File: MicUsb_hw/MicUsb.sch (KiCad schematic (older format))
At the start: 29 parts

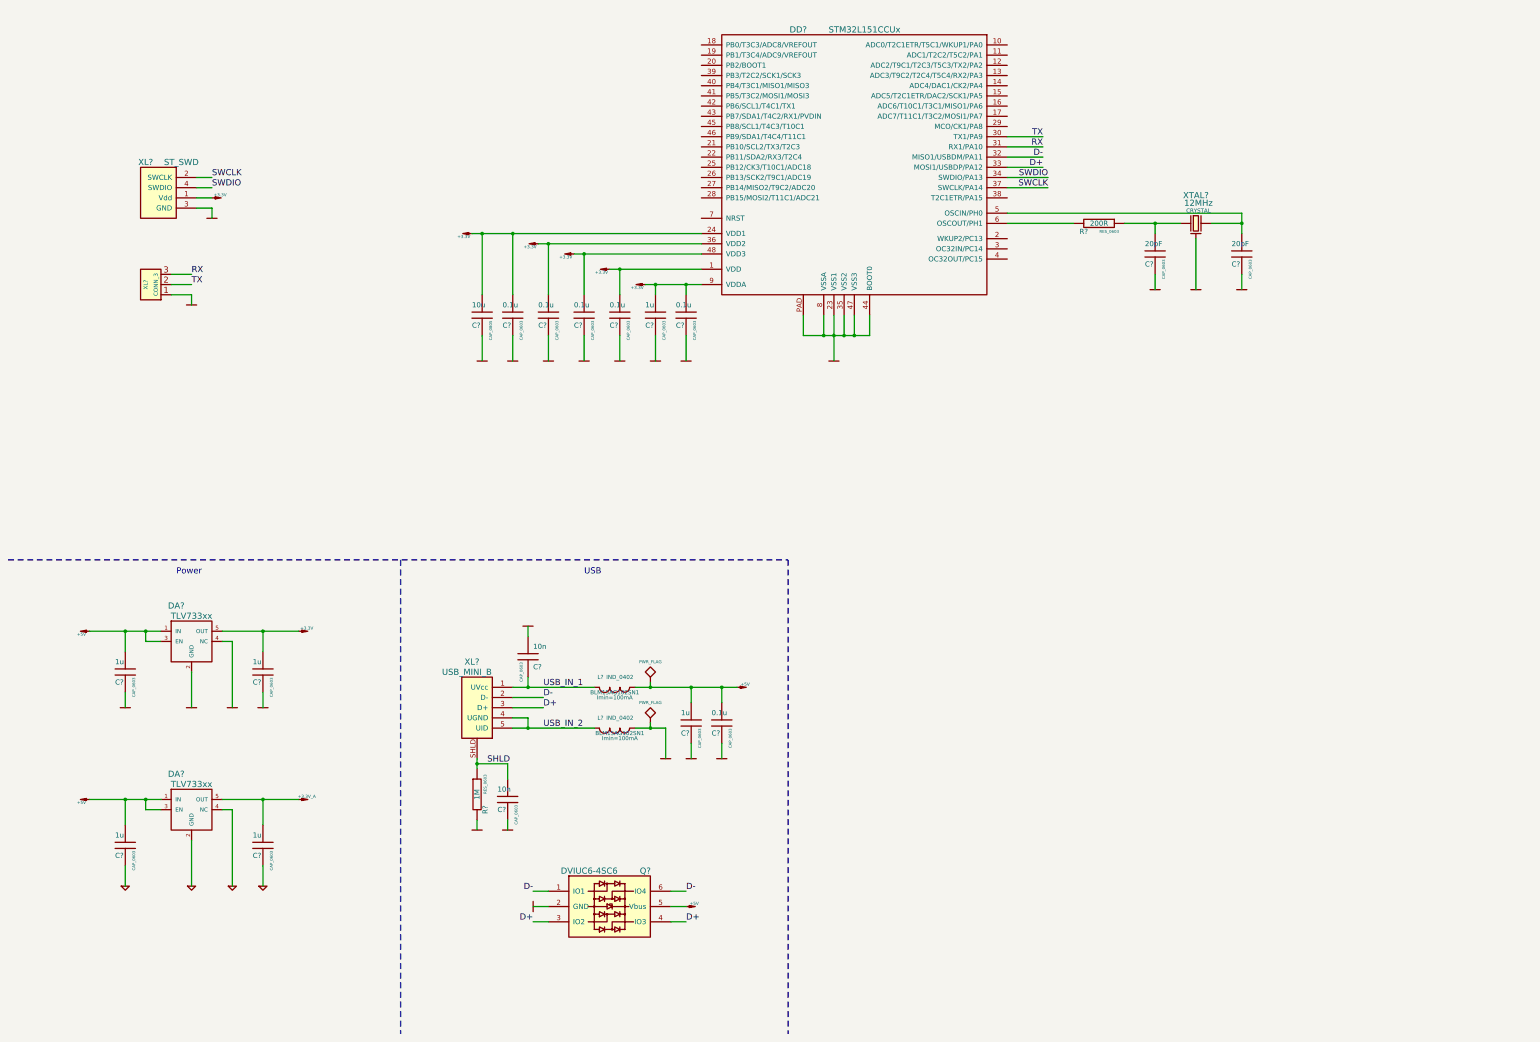
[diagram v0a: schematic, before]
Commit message: sch update, i need answers!
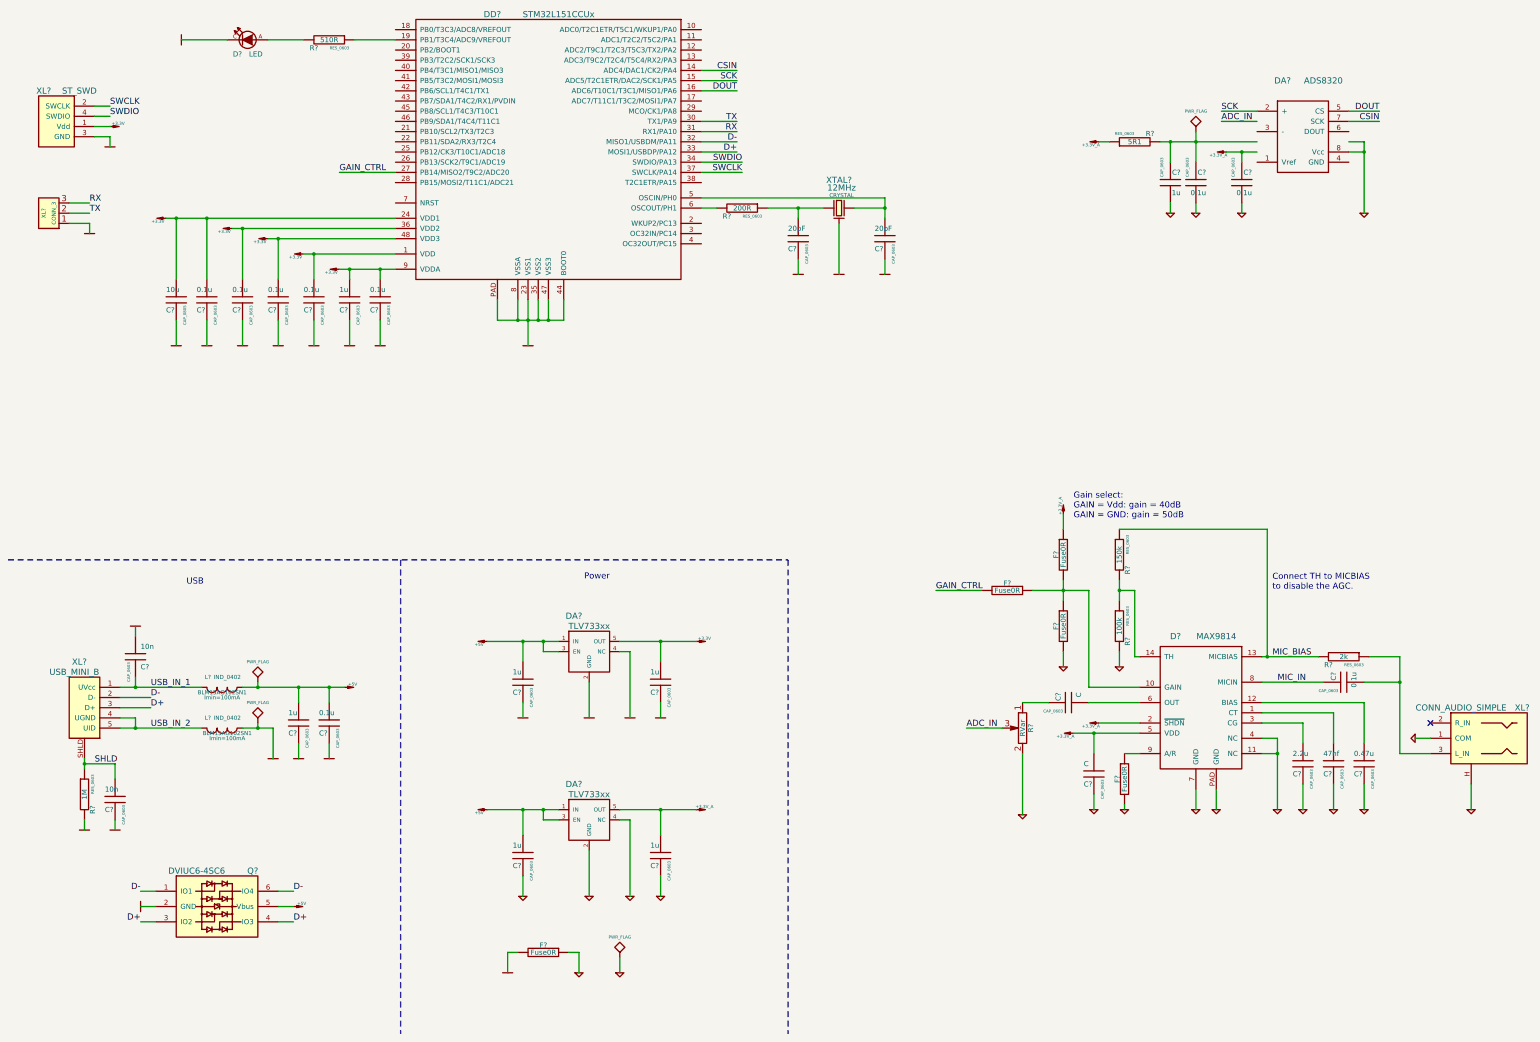
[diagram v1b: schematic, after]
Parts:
- added C?: 2.2u, CAP_0603, symbol C
- added C?: 47nf, CAP_0603, symbol C
- added C?: 0.47u, CAP_0603, symbol C
- added C? (x3): 0.1u, CAP_0603, symbol C
- added C? (x2): C, CAP_0603, symbol C
- added C?: 1u, CAP_0603, symbol C
- added D?: LED, symbol LED
- added D?: MAX9814, symbol MAX9814
- added DA?: ADS8320, symbol ADS8320
- added F? (x5): Fuse0R, symbol Fuse0R
- added R?: 510R, RES_0603, symbol R
- added R?: 2k, RES_0603, symbol R
- added R?: 100k, RES_0603, symbol R
- added R?: 150k, RES_0603, symbol R
- added R?: RVar, symbol RVar
- added R?: 5R1, RES_0603, symbol R
- added XL?: CONN_AUDIO_SIMPLE, symbol CONN_AUDIO_SIMPLE
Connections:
- net +3.3V_A: now also C?.1, C?.2, D?.2 (~SHDN), D?.5 (VDD), F?.1, R?.1
- net AGND: now also C?.1, C?.1, C?.1, C?.2, C?.2, C?.2, C?.2, D?.11 (NC), D?.4 (NC), D?.7 (GND), D?.PAD (GND), DA?.8 (Vcc), F?.1, F?.2, F?.2, R?.2, R?.2, XL?.1 (COM), XL?.H
- net GND: now also D?.C, F?.2
- net CSIN: now reaches DD?.14 (ADC4/DAC1/CK2/PA4)
- net CSIN: now also DA?.7 (SCK)
- net SCK: now reaches DD?.15 (ADC5/T2C1ETR/DAC2/SCK1/PA5)
- net SCK: now also DA?.2 (+)
- net DOUT: now reaches DD?.16 (ADC6/T10C1/T3C1/MISO1/PA6)
- net DOUT: now also DA?.5 (CS)
- net at DD?.19 (PB1/T3C4/ADC9/VREFOUT): now also R?.1
- net GAIN_CTRL: now reaches DD?.27 (PB14/MISO2/T9C2/ADC20)
- net GAIN_CTRL: now also F?.2
- new net: D?.A, R?.2
- new net: C?.1, D?.1 (CT)
- new net: D?.10 (GAIN), F?.1, F?.1, F?.2
- new net: C?.1, D?.12 (BIAS)
- new net: D?.14 (TH), R?.1, R?.2
- new net: C?.1, D?.3 (CG)
- new net: C?.1, D?.6 (OUT)
- new net: D?.9 (A/R), F?.1
- new net: C?.1, R?.1, XL?.3 (L_IN)
- new net: C?.2, R?.1
- new net: C?.2, C?.2, R?.2
- new net ADC_IN: R?.3
- new net MIC_BIAS: D?.13 (MICBIAS), R?.1, R?.2
- new net MIC_IN: C?.2, D?.8 (MICIN)
- no-connect marks 0 -> 1
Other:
- note added: "Connect TH to MICBIAS\nto disable the AGC."
- note added: "Gain select:\nGAIN = Vdd: gain = 40dB\nGAIN = GND: gain = 50dB"
- moved on the sheet: C?, DA?, DD?, L?, Q?, R?, XL?, XTAL?

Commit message: * ADS
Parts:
- removed C?: C, CAP_0603, symbol C
- removed DA?: ADS8320, symbol ADS8320
- added DA?: ADS8320, symbol ADS8320
- XL?: symbol USB_MINI_B -> USB_MINI_B-RESCUE-MicUsb
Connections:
- net +3.3V_A: now also DA?.1 (Vref)
- net ADC_IN: now also DA?.2 (+)
- net AGND: now also DA?.3 (-), DA?.4 (GND)
- net CSIN: now also DA?.5 (CS)
- net DOUT: now also DA?.6 (DOUT)
- net SCK: now also DA?.7 (SCK)
- net at D?.6 (OUT): now also R?.1
- net at C?.2, C?.2, R?.2: now also DA?.8 (Vcc)
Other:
- moved on the sheet: C?, D?, DD?, F?, R?, XL?, XTAL?
